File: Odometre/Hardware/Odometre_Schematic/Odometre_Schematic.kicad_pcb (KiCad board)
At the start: 2 copper layers, 83.2 x 61.6 mm, 35 parts, among them IC1 STM32C092FCP6, J1 Conn_01x03_Pin, J2 Conn_01x03_Pin, J3 Conn_Alim, J4 Conn_Laser1, J5 Conn_Laser2, J6 Conn_SWD, J7 Conn_01x06_Pin, U1 MCP2562-E-SN, U2 LM1117DT-3.3, U3 LM1117DT-5.0

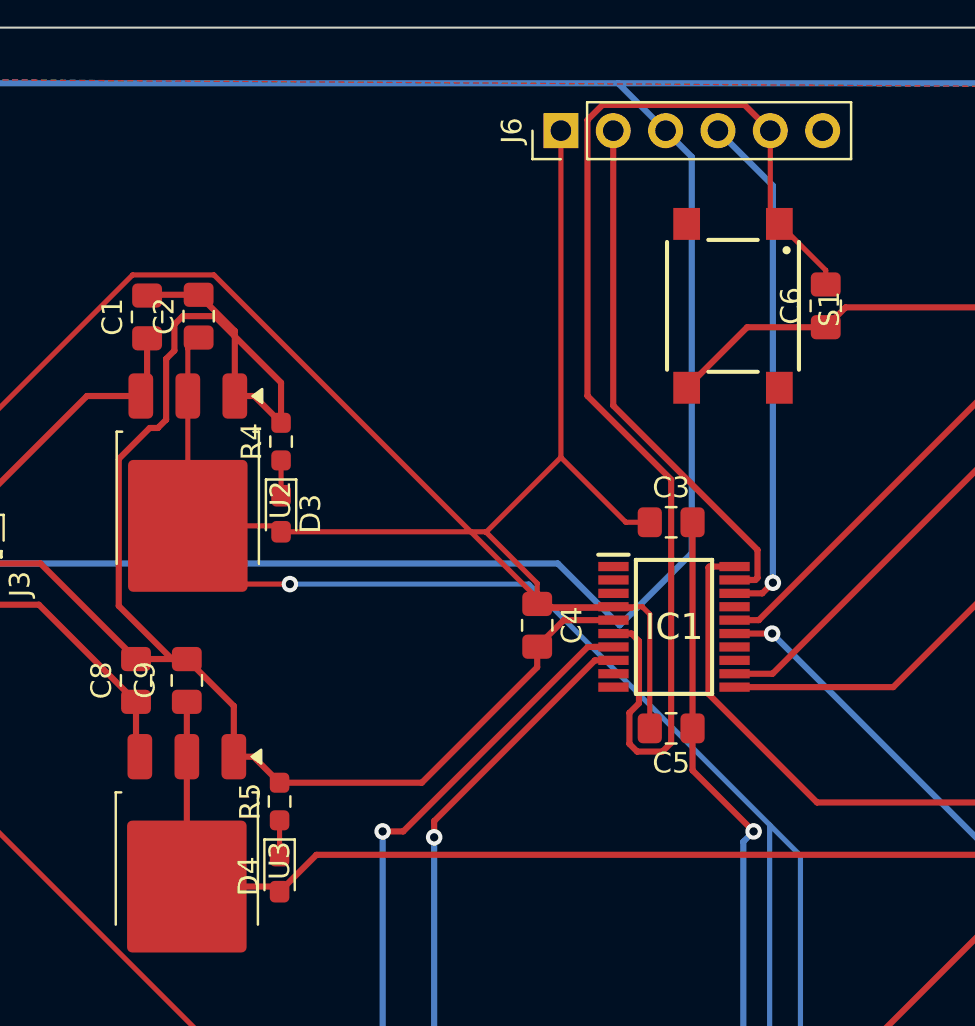
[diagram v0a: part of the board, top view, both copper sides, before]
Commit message: Modification PCB pour impression
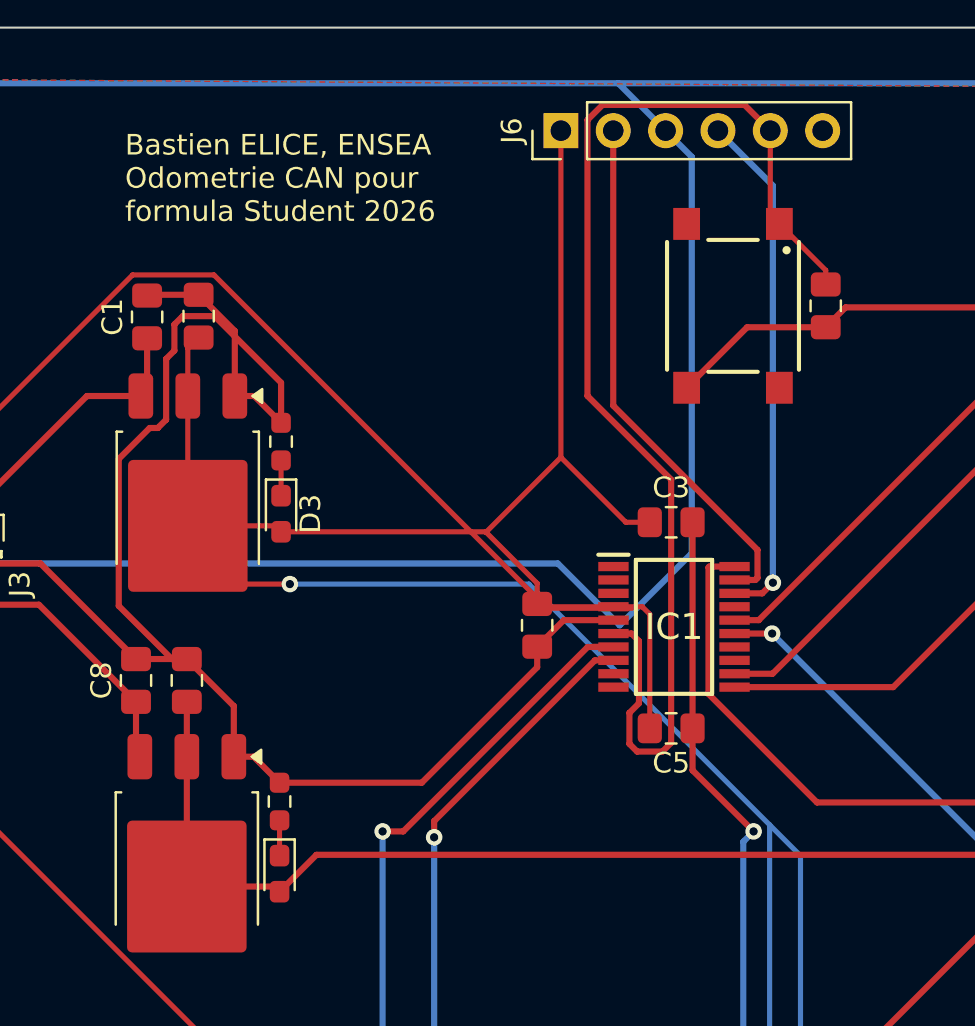
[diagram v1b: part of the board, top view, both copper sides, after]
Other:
- board text added: "Bastien ELICE, ENSEA Odometrie CAN pour formula Student 2026"
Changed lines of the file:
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@@
 			(outputformat 1)
 			(mirror no)
-			(drillshape 1)
+			(drillshape 0)
 			(scaleselection 1)
-			(outputdirectory "")
+			(outputdirectory "fichier_de_fabrication/")
 		)
 	)
@@
 			(at 0 -1.43 90)
 			(layer "F.SilkS")
+			(hide yes)
 			(effects
 				(font
@@
 			(at 0 -1.68 90)
 			(layer "F.SilkS")
+			(hide yes)
 			(effects
 				(font
@@
 			(at 0.125 1.5 90)
 			(layer "F.SilkS")
+			(hide yes)
 			(effects
 				(font
@@
 			(at 0.02 -2.03 90)
 			(layer "F.SilkS")
+			(hide yes)
 			(effects
 				(font
@@
 			(at 0 -1.43 90)
 			(layer "F.SilkS")
+			(hide yes)
 			(effects
 				(font
@@
 			(at 0.153 -4.6759 90)
 			(layer "F.SilkS")
+			(hide yes)
 			(effects
 				(font
@@
 			(at 0 -4.5 90)
 			(layer "F.SilkS")
+			(hide yes)
 			(effects
 				(font
@@
 			(at 0 -1.68 90)
 			(layer "F.SilkS")
+			(hide yes)
 			(effects
 				(font
@@
 			(at 0 -1.68 90)
 			(layer "F.SilkS")
+			(hide yes)
 			(effects
 				(font
@@
 			(at 0 -4.5 90)
 			(layer "F.SilkS")
+			(hide yes)
 			(effects
 				(font
@@
 		(layer "Edge.Cuts")
 	)
+	(gr_text "Bastien ELICE, ENSEA\nOdometrie CAN pour\nformula Student 2026"
+		(at 126 68.5 0)
+		(layer "F.SilkS")
+		(effects
+			(font
+				(size 1 1)
+				(thickness 0.15)
+			)
+			(justify left bottom)
+		)
+	)
 	(segment

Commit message: k
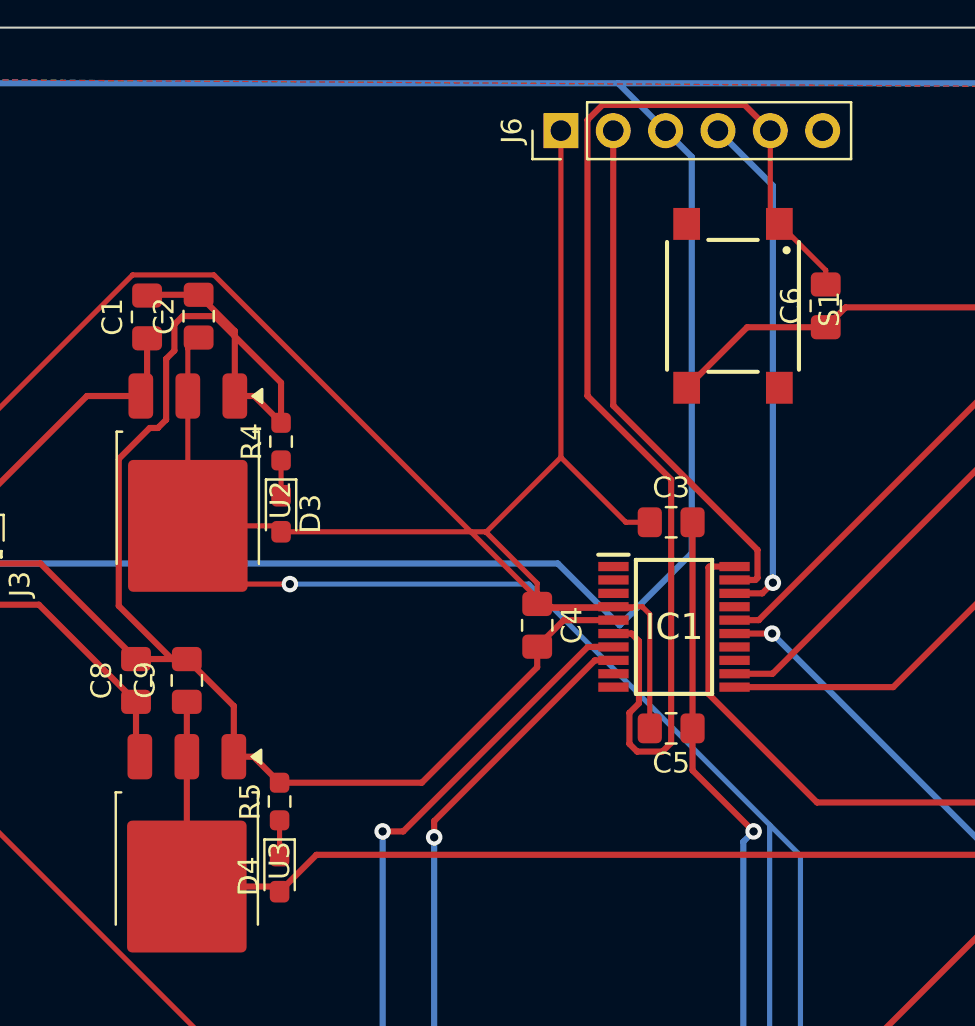
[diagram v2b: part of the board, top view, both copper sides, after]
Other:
- board text removed: "Bastien ELICE, ENSEA Odometrie CAN pour formula Student 2026"
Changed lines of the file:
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@@
 			(outputformat 1)
 			(mirror no)
-			(drillshape 0)
+			(drillshape 1)
 			(scaleselection 1)
-			(outputdirectory "fichier_de_fabrication/")
+			(outputdirectory "")
 		)
 	)
@@
 			(at 0 -1.43 90)
 			(layer "F.SilkS")
-			(hide yes)
 			(effects
 				(font
@@
 			(at 0 -1.68 90)
 			(layer "F.SilkS")
-			(hide yes)
 			(effects
 				(font
@@
 			(at 0.125 1.5 90)
 			(layer "F.SilkS")
-			(hide yes)
 			(effects
 				(font
@@
 			(at 0.02 -2.03 90)
 			(layer "F.SilkS")
-			(hide yes)
 			(effects
 				(font
@@
 			(at 0 -1.43 90)
 			(layer "F.SilkS")
-			(hide yes)
 			(effects
 				(font
@@
 			(at 0.153 -4.6759 90)
 			(layer "F.SilkS")
-			(hide yes)
 			(effects
 				(font
@@
 			(at 0 -4.5 90)
 			(layer "F.SilkS")
-			(hide yes)
 			(effects
 				(font
@@
 			(at 0 -1.68 90)
 			(layer "F.SilkS")
-			(hide yes)
 			(effects
 				(font
@@
 			(at 0 -1.68 90)
 			(layer "F.SilkS")
-			(hide yes)
 			(effects
 				(font
@@
 			(at 0 -4.5 90)
 			(layer "F.SilkS")
-			(hide yes)
 			(effects
 				(font
@@
 		(layer "Edge.Cuts")
 	)
-	(gr_text "Bastien ELICE, ENSEA\nOdometrie CAN pour\nformula Student 2026"
-		(at 126 68.5 0)
-		(layer "F.SilkS")
-		(effects
-			(font
-				(size 1 1)
-				(thickness 0.15)
-			)
-			(justify left bottom)
-		)
-	)
 	(segment
